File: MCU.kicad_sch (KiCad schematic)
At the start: 28 parts, among them IC1 RP2040, J1 USB_C_Receptacle_USB2.0, SW1 SW_SPST, SW2 SW_SPST, U1 NCP163ASN330T1G, U3 W25X40CLSN, Y1 Crystal_GND24_Small

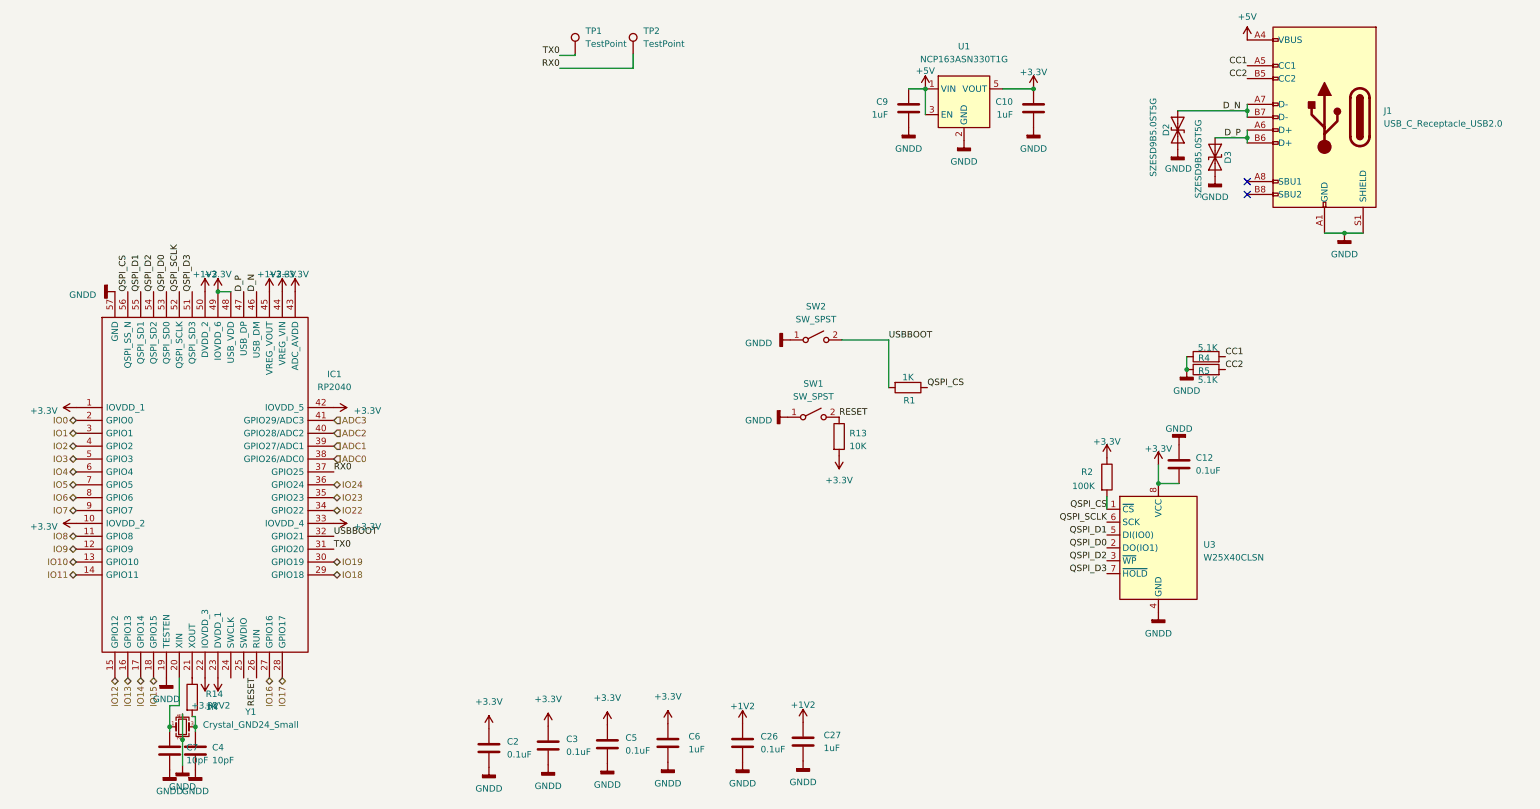
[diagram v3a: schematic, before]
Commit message: sarted samd21 layout
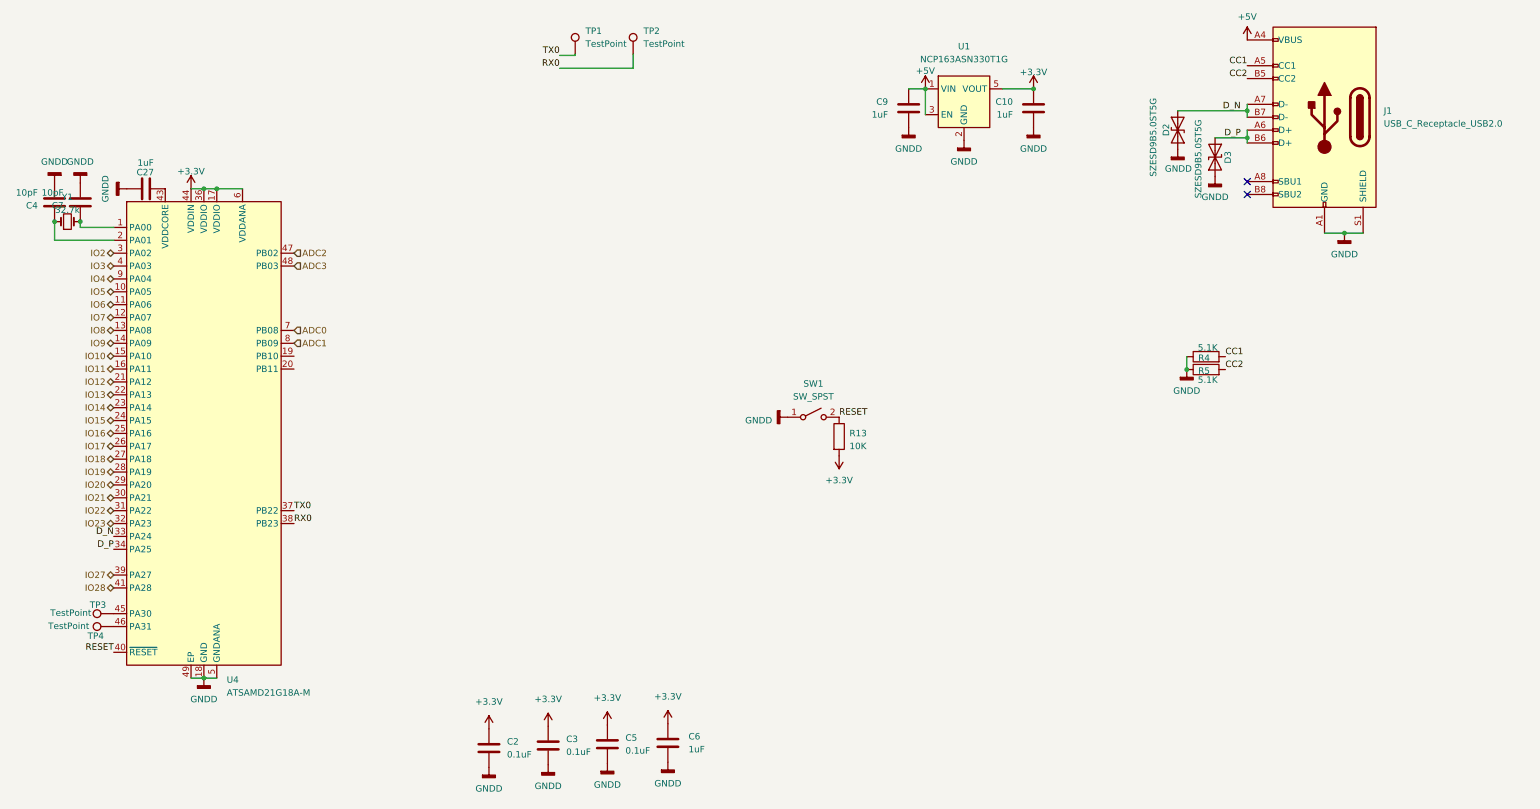
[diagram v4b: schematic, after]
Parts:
- removed C12, C26: 0.1uF, Capacitor_SMD:C_0402_1005Metric, symbol Device:C
- removed IC1: RP2040, RP2040:QFN40P700X700X90-57N-D, symbol RP2040:RP2040
- removed R1, R14: 1K, Resistor_SMD:R_0402_1005Metric, symbol Device:R
- removed R2: 100K, Resistor_SMD:R_0402_1005Metric, symbol Device:R
- removed SW2: SW_SPST, Button_Switch_SMD:SW_SPST_B3U-1000P-B, symbol Switch:SW_SPST
- removed U3: W25X40CLSN, Package_SO:SOIC-8_3.9x4.9mm_P1.27mm, symbol Memory_Flash:W25X40CLSN
- removed Y1: Crystal_GND24_Small, Crystal:Crystal_SMD_2520-4Pin_2.5x2.0mm, symbol Device:Crystal_GND24_Small
- added TP3, TP4: TestPoint, TestPoint:TestPoint_Pad_2.0x2.0mm, symbol Connector:TestPoint
- added U4: ATSAMD21G18A-M, Package_DFN_QFN:QFN-48-1EP_7x7mm_P0.5mm_EP5.15x5.15mm, symbol MCU_Microchip_SAMD:ATSAMD21G18A-M
- added Y1: 32.7k, Crystal:Crystal_SMD_2012-2Pin_2.0x1.2mm, symbol Device:Crystal_Small
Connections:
- net +3.3V: now also U4.17 (VDDIO), U4.36 (VDDIO), U4.44 (VDDIN), U4.6 (VDDANA)
- net ADC0: now also U4.7 (PB08)
- net ADC1: now also U4.8 (PB09)
- net ADC2: now also U4.47 (PB02)
- net ADC3: now also U4.48 (PB03)
- net D_N: now also U4.33 (PA24)
- net D_P: now also U4.34 (PA25)
- net GNDD: now also U4.18 (GND), U4.35 (GND), U4.42 (GND), U4.49 (EP), U4.5 (GNDANA)
- net IO10: now also U4.15 (PA10)
- net IO11: now also U4.16 (PA11)
- net IO12: now also U4.21 (PA12)
- net IO13: now also U4.22 (PA13)
- net IO14: now also U4.23 (PA14)
- net IO15: now also U4.24 (PA15)
- net IO16: now also U4.25 (PA16)
- net IO17: now also U4.26 (PA17)
- net IO18: now also U4.27 (PA18)
- net IO19: now also U4.28 (PA19)
- net IO2: now also U4.3 (PA02)
- net IO22: now also U4.31 (PA22)
- net IO23: now also U4.32 (PA23)
- net IO3: now also U4.4 (PA03)
- net IO4: now also U4.9 (PA04)
- net IO5: now also U4.10 (PA05)
- net IO6: now also U4.11 (PA06)
- net IO7: now also U4.12 (PA07)
- net IO8: now also U4.13 (PA08)
- net IO9: now also U4.14 (PA09)
- net RESET: now also U4.40 (~{RESET})
- net RX0: now also U4.38 (PB23)
- net TX0: now also U4.37 (PB22)
- net at C7.1: now also U4.1 (PA00), Y1.2
- net at C4.1: now also U4.2 (PA01), Y1.1
- net +1V2: no longer names the net of C27.1
- net +1V2: now also U4.43 (VDDCORE)
- new net: TP3.1, U4.45 (PA30)
- new net: TP4.1, U4.46 (PA31)
- new net IO20: U4.29 (PA20)
- new net IO21: U4.30 (PA21)
- new net IO27: U4.39 (PA27)
- new net IO28: U4.41 (PA28)
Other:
- moved on the sheet: C27, C4, C7
